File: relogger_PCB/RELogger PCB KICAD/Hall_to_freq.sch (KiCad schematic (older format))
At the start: 4 parts, among them P26 JMP_HALL, U6 LM393

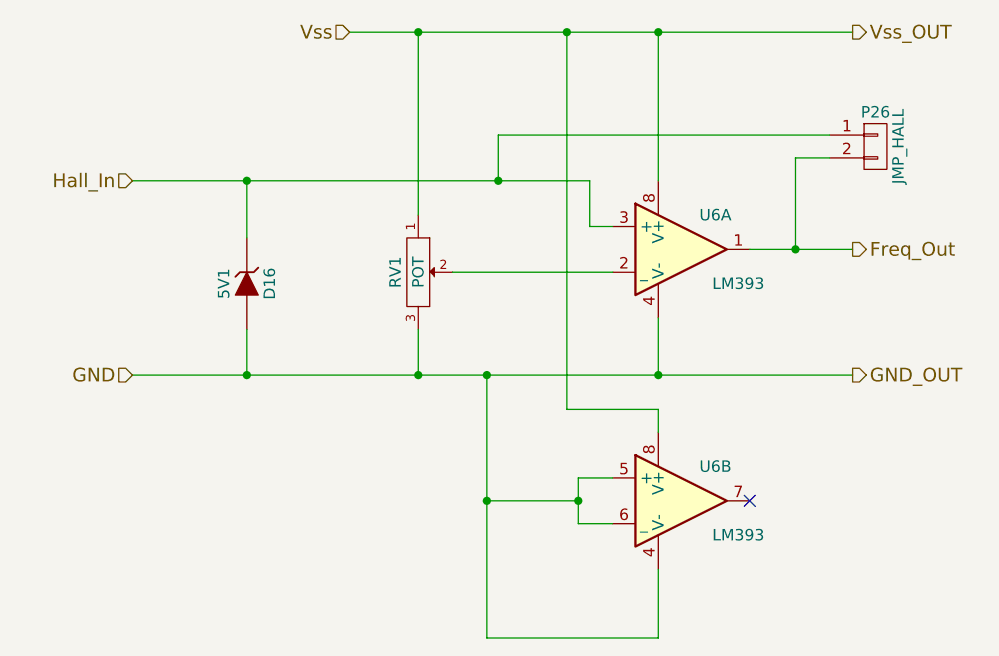
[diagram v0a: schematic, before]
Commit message: Update of schematic
By ML
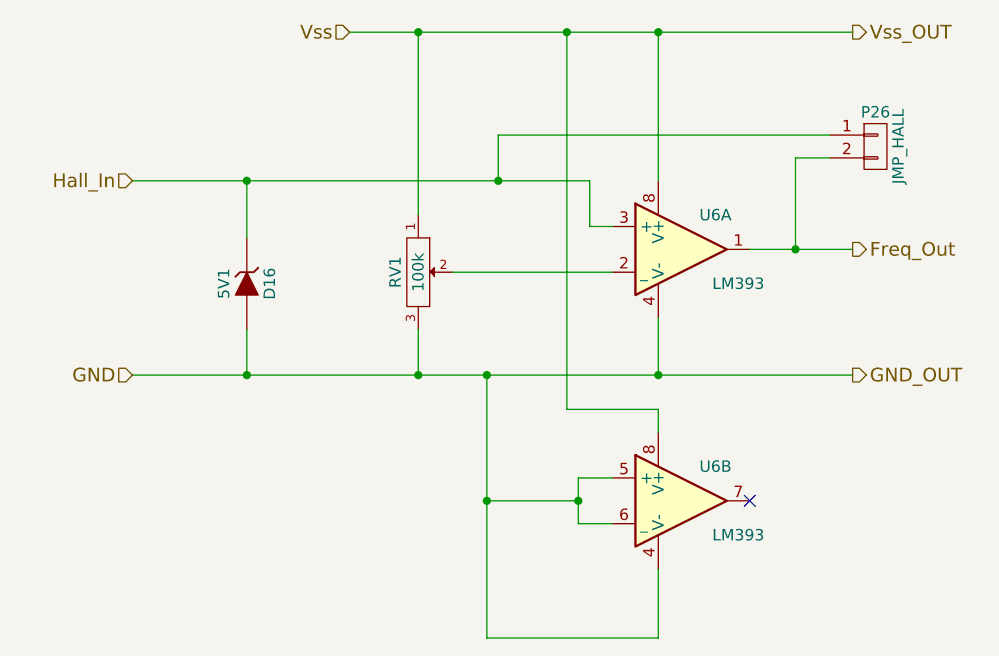
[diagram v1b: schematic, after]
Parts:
- RV1: value POT -> 100k
- U6: Description (none) -> Op Amp; Manufacturer (none) -> ON Semi; Manufacturer Part No (none) -> LM393NG; Supplier 1 (none) -> RS; Supplier 1 Cost (none) -> 0.25; Supplier 1 Part No (none) -> 463-870
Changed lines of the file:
@@
 LIBS:matts_components
 LIBS:linear2
-LIBS:ds3231
-LIBS:micro_sd
 LIBS:RELogger_PCB_v1-cache
 EELAYER 25 0
@@
 F 1 "LM393" H 6950 3100 50  0000 C CNN
 F 2 "" H 6700 3250 50  0000 C CNN
-F 3 "" H 6700 3250 50  0000 C CNN
+F 3 "http://docs-europe.electrocomponents.com/webdocs/13e4/0900766b813e452a.pdf" H 6700 3250 50  0001 C CNN
+F 4 "~" H 6700 3250 60  0000 C CNN "Notes"
+F 5 "Op Amp" H 6700 3250 60  0001 C CNN "Description"
+F 6 "ON Semi" H 6700 3250 60  0001 C CNN "Manufacturer"
+F 7 "LM393NG" H 6700 3250 60  0001 C CNN "Manufacturer Part No"
+F 8 "RS" H 6700 3250 60  0001 C CNN "Supplier 1"
+F 9 "463-870" H 6700 3250 60  0001 C CNN "Supplier 1 Part No"
+F 10 "0.25" H 6700 3250 60  0001 C CNN "Supplier 1 Cost"
+F 11 "~" H 6700 3250 60  0001 C CNN "Supplier 2"
+F 12 "~" H 6700 3250 60  0001 C CNN "Supplier 2 Part No"
+F 13 "~" H 6700 3250 60  0001 C CNN "Supplier 2 Cost"
 	1    6700 3250
 	1    0    0    -1
@@
 P 5550 3350
 F 0 "RV1" H 5550 3250 50  0000 C CNN
-F 1 "POT" H 5550 3350 50  0000 C CNN
+F 1 "100k" H 5550 3350 50  0000 C CNN
 F 2 "" H 5550 3350 50  0000 C CNN
 F 3 "" H 5550 3350 50  0000 C CNN
